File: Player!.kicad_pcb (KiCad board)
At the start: 2 copper layers, 95.2 x 38.1 mm, 25 parts, among them J1 USB4085-GF-A_REVA4, SW1 SW_Push, SW2 SW_Push, SW3 SW_Push, SW4 SW_Push, SW5 RotaryEncoder_Switch

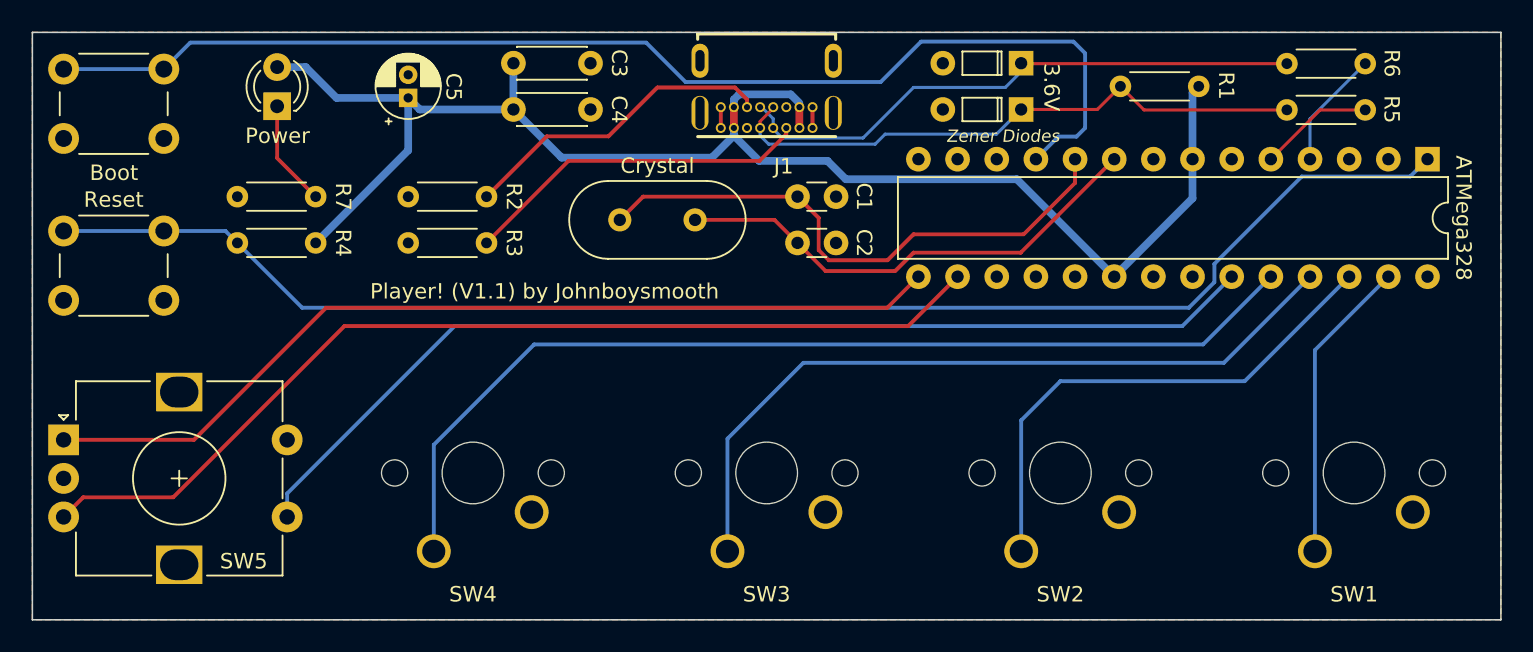
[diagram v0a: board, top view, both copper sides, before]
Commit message: Updating PCB and Models for Case
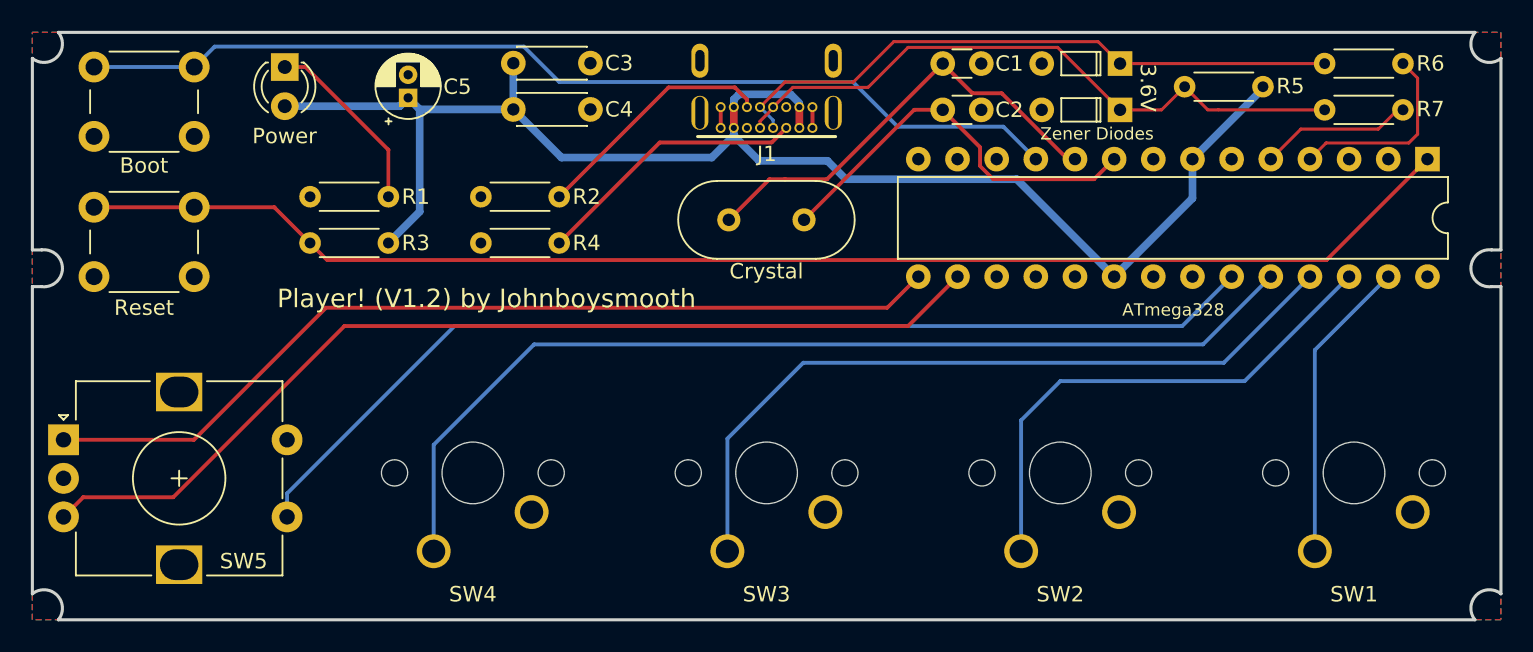
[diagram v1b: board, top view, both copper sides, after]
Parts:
- moved C1 12.8 mm to (59.0, 2.02)
- moved C2 12.8 mm to (59.0, 5.02)
- moved Crystal1 7.07 mm to (45.2, 12.2)
- moved DN1 6.42 mm to (70.5, 2.02)
- moved DP1 6.42 mm to (70.5, 5.02)
- moved R2 4.72 mm to (34.2, 10.7)
- moved R4 4.72 mm to (34.2, 13.7)
- moved R1 4.72 mm to (23.1, 10.7)
- moved R3 4.72 mm to (23.1, 13.7)
- moved R5 4.17 mm to (79.8, 3.52)
- moved Power 2.59 mm to (16.4, 2.25), turned to -90 degrees
- moved Reset 2.50 mm to (4.00, 11.3)
- moved R6 2.45 mm to (83.8, 2.02)
- moved R7 2.45 mm to (83.8, 5.02)
- moved Boot 1.97 mm to (4.00, 2.25)
- renumbered ATMega328 to ATmega328, R7 to R1, R4 to R3, R3 to R4, R1 to R5, R5 to R7
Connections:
- J1 pad P1: (no net) -> GND
- J1 pad P2: (no net) -> GND
- J1 pad P3: (no net) -> GND
- J1 pad P4: (no net) -> GND
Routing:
- net /BOOT: track 78.3 -> 64.7 mm
- net /XTAL2: track 36.7 -> 29.2 mm
- net /XTAL1: track 31.6 -> 26.2 mm
- net /CC1: track 23.0 -> 17.8 mm
- net /LED: track 6.90 -> 12.0 mm
- net D+: track 7.68 -> 12.6 mm
- net /CC2: track 20.6 -> 15.9 mm
- net /RST: track 95.2 -> 90.6 mm
- net /DN: track 38.8 -> 41.6 mm
- net /DP: track 37.7 -> 40.3 mm
- net D-: track 7.44 -> 9.55 mm
- net +5V: track 99.2 -> 97.4 mm
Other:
- outline, holes or cut-outs redrawn
- board text added: "Player! (V1.2) by Johnboysmooth"
- board text removed: "Player! (V1.1) by Johnboysmooth"
